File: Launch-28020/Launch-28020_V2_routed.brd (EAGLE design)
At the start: 74.2 x 45.1 mm, 26 parts, among them X1 C-GRID-06-74099, X2 C-GRID-04-74099, X3 C-GRID-06-74099, X4 C-GRID-08-74099, X5 C-GRID-07-74099, X6 C-GRID-03-74099, X7 C-GRID-03-74099, X8 C-GRID-03-74099, X9 C-GRID-03-74099

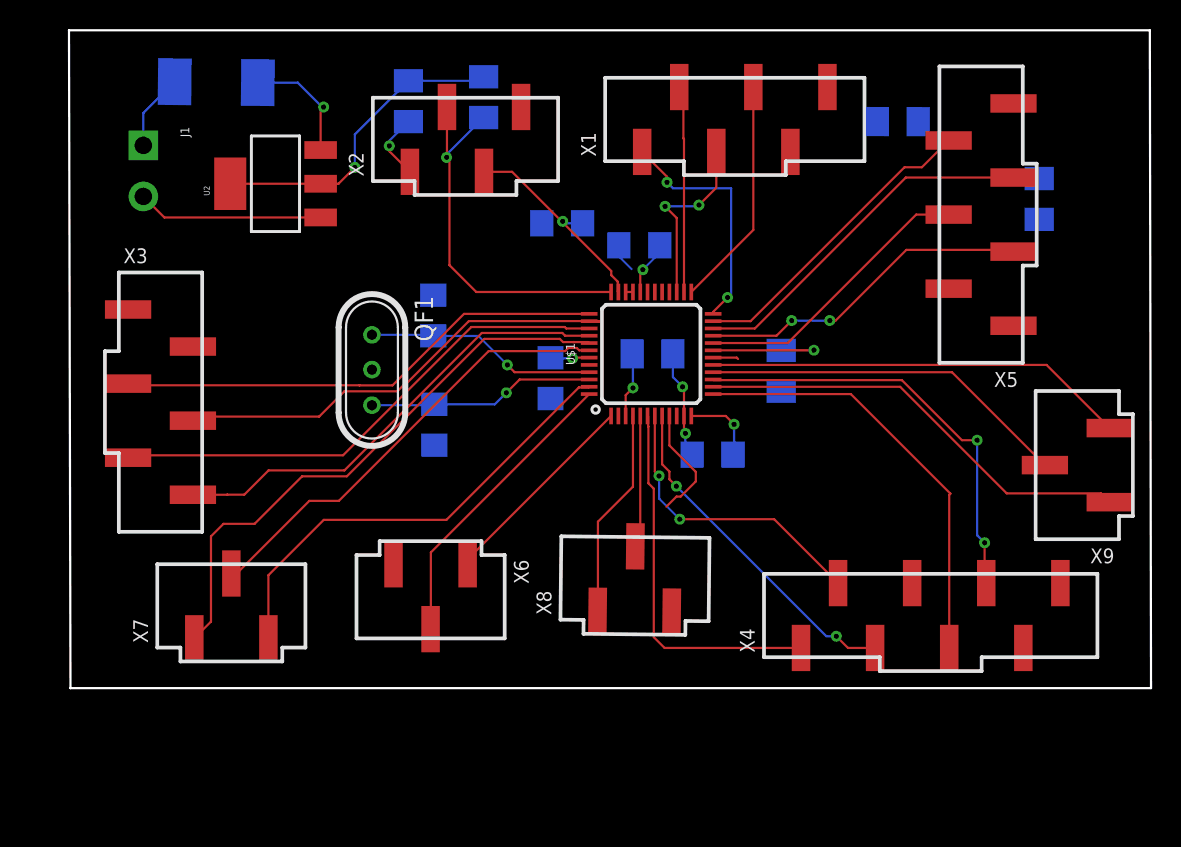
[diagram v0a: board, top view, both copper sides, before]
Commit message: Updated Layout
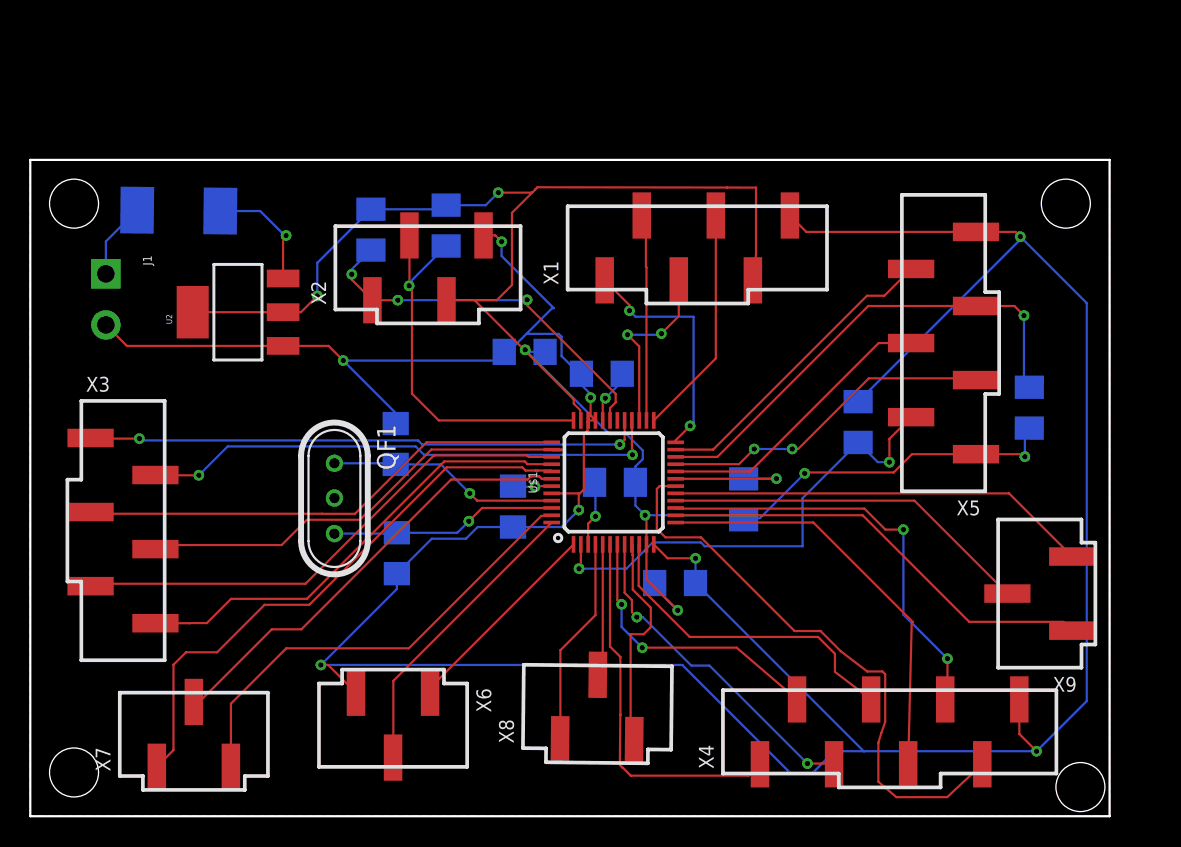
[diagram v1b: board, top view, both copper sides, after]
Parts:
- moved R2 21.6 mm to (68.5, 28.0), turned to 90.1 degrees
- moved R1 19.7 mm to (56.8, 27.0)
- moved R5 9.18 mm to (40.1, 22.9)
- moved X1 9.18 mm to (45.7, 39.0)
- moved D1 9.18 mm to (10.2, 41.5)
- moved R6 9.18 mm to (28.5, 40.5)
- moved U2 9.18 mm to (14.2, 34.6)
- moved X5 9.18 mm to (62.6, 32.4)
- moved X8 9.18 mm to (38.9, 7.47)
- moved C1 9.18 mm to (25.1, 18.0)
- moved C7 9.18 mm to (44.2, 16.0)
- moved C8 9.18 mm to (25.1, 25.5)
- moved C9 9.18 mm to (33.9, 31.8)
- moved R3 9.18 mm to (48.9, 21.7)
- moved U$1 9.18 mm to (40.0, 22.9)
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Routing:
- net GND: track 20.5 -> 239.9 mm, vias 1 -> 8
- net VDD: track 43.9 -> 130.5 mm, vias 4 -> 7
- net PWM1H: track 0.00 -> 38.3 mm, vias 0 -> 2
- net ADC_B7: track 1.75 -> 39.6 mm
- net PWM1L: track 0.00 -> 36.2 mm, vias 0 -> 2
- net TRST: track 0.00 -> 33.0 mm, vias 0 -> 2
- net ADC_A0: track 0.00 -> 22.6 mm
- net I2C_SDA: track 4.57 -> 26.1 mm, vias 1 -> 3
- net TDO: track 24.9 -> 33.5 mm, vias 0 -> 1
- net AIO2: track 8.19 -> 15.4 mm
- net ADC_B1: track 29.7 -> 28.9 mm
- net ADC_A3: track 20.5 -> 19.7 mm
- net ADC_B3: track 29.9 -> 29.2 mm
- added copper zone on layer 1, net N$2
- added copper zone on layer 16, net N$9
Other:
- board size 74.2 x 45.1 mm -> 74 x 45 mm
